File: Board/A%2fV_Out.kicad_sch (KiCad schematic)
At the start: 21 parts, among them J1 HDMI_A

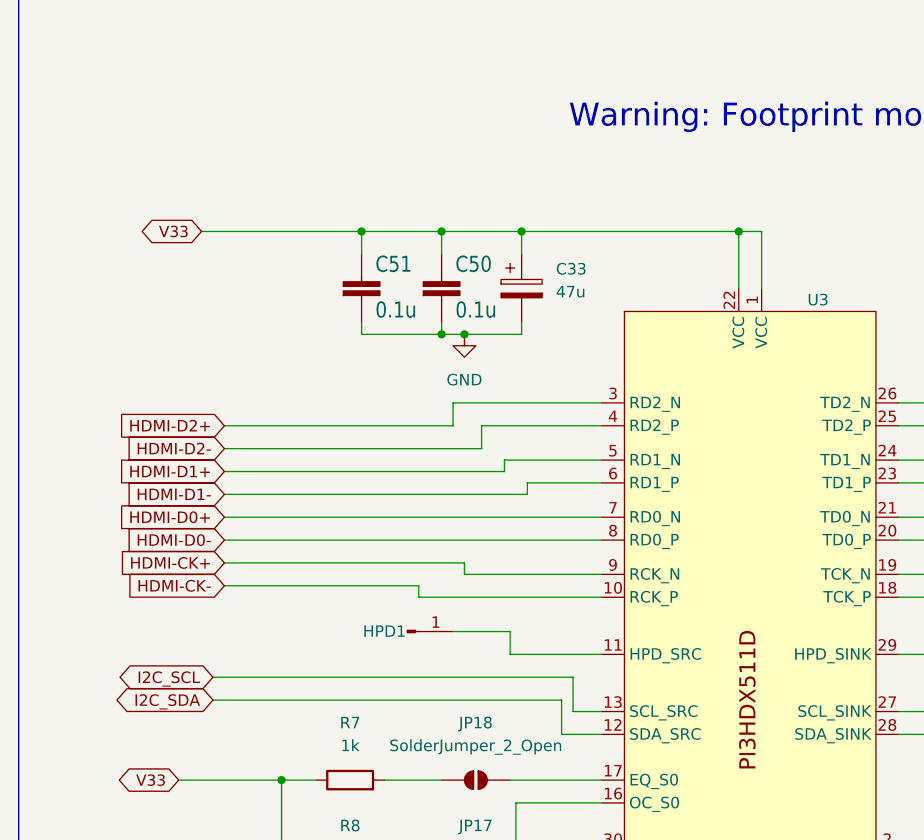
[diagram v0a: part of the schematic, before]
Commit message: layout work
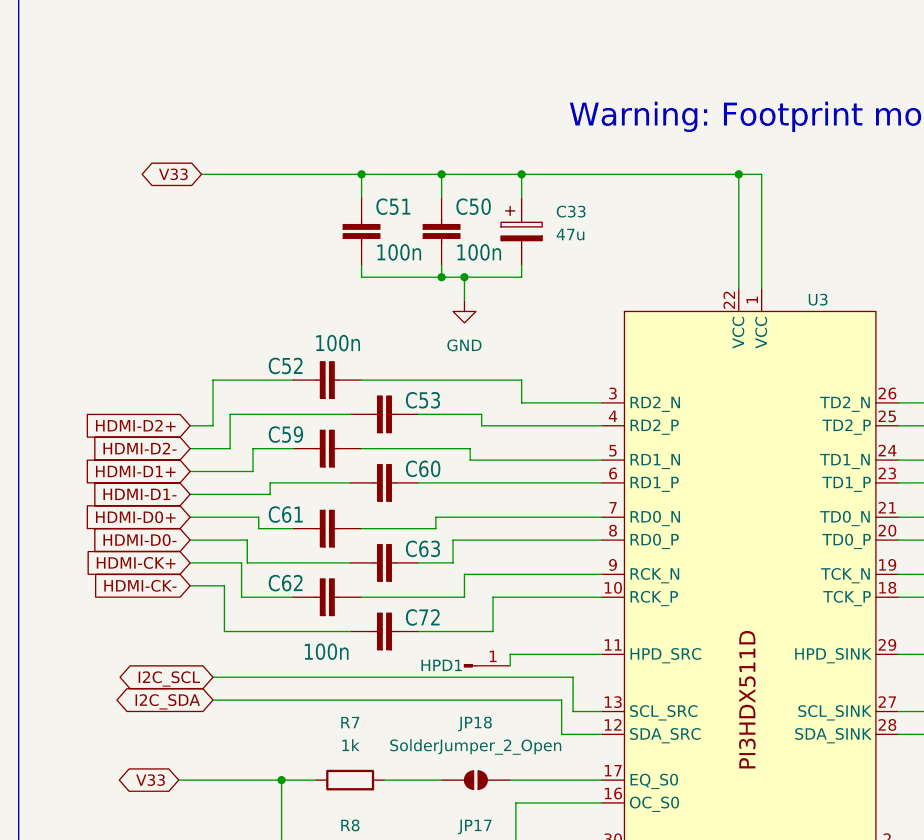
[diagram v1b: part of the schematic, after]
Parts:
- added C52, C53, C59, C60, C61, C62, C63, C72: 100n, Capacitor_SMD:C_0603_1608Metric_Pad1.08x0.95mm_HandSolder, symbol csa_ultracpu-eagle-import:C-EUC0603
- C50, C51: value 0.1u -> 100n; footprint csa_ultracpu:C0603 -> Capacitor_SMD:C_0603_1608Metric_Pad1.08x0.95mm_HandSolder
- U3: value ~ -> (none)
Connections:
- net HDMI-CK+: now also C62.1; no longer U3.9 (RCK_N)
- net HDMI-CK-: now also C72.1; no longer U3.10 (RCK_P)
- net HDMI-D0+: now also C61.1; no longer U3.7 (RD0_N)
- net HDMI-D0-: now also C63.1; no longer U3.8 (RD0_P)
- net HDMI-D1+: now also C59.1; no longer U3.5 (RD1_N)
- net HDMI-D1-: now also C60.1; no longer U3.6 (RD1_P)
- net HDMI-D2+: now also C52.1; no longer U3.3 (RD2_N)
- net HDMI-D2-: now also C53.1; no longer U3.4 (RD2_P)
- new net: C53.2, U3.4 (RD2_P)
- new net: C61.2, U3.7 (RD0_N)
- new net: C62.2, U3.9 (RCK_N)
- new net: C63.2, U3.8 (RD0_P)
- new net: C72.2, U3.10 (RCK_P)
- new net: C52.2, U3.3 (RD2_N)
- new net: C59.2, U3.5 (RD1_N)
- new net: C60.2, U3.6 (RD1_P)
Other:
- moved on the sheet: C33, C50, C51, HPD1
